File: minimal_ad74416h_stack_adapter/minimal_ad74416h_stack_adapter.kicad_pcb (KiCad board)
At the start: 2 copper layers, 5.1 x 5.1 mm, 0 parts

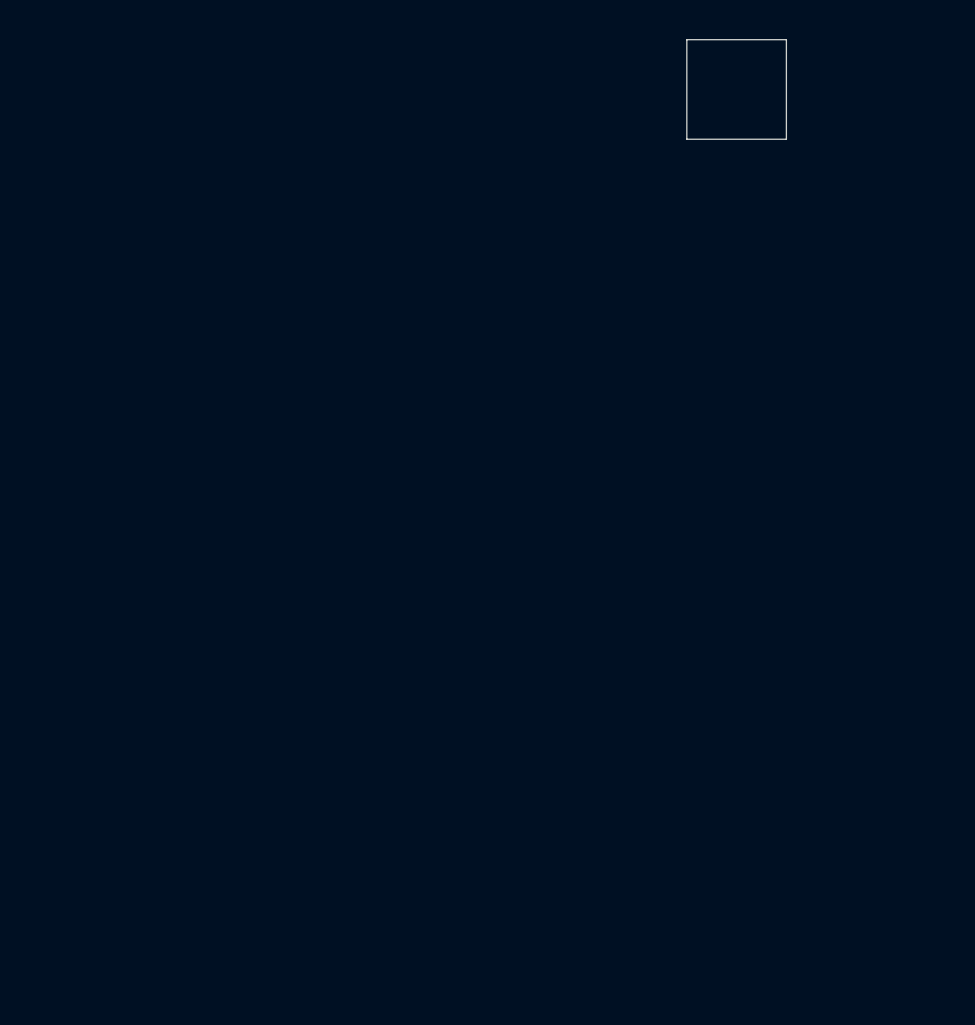
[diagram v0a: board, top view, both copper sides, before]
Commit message: backup
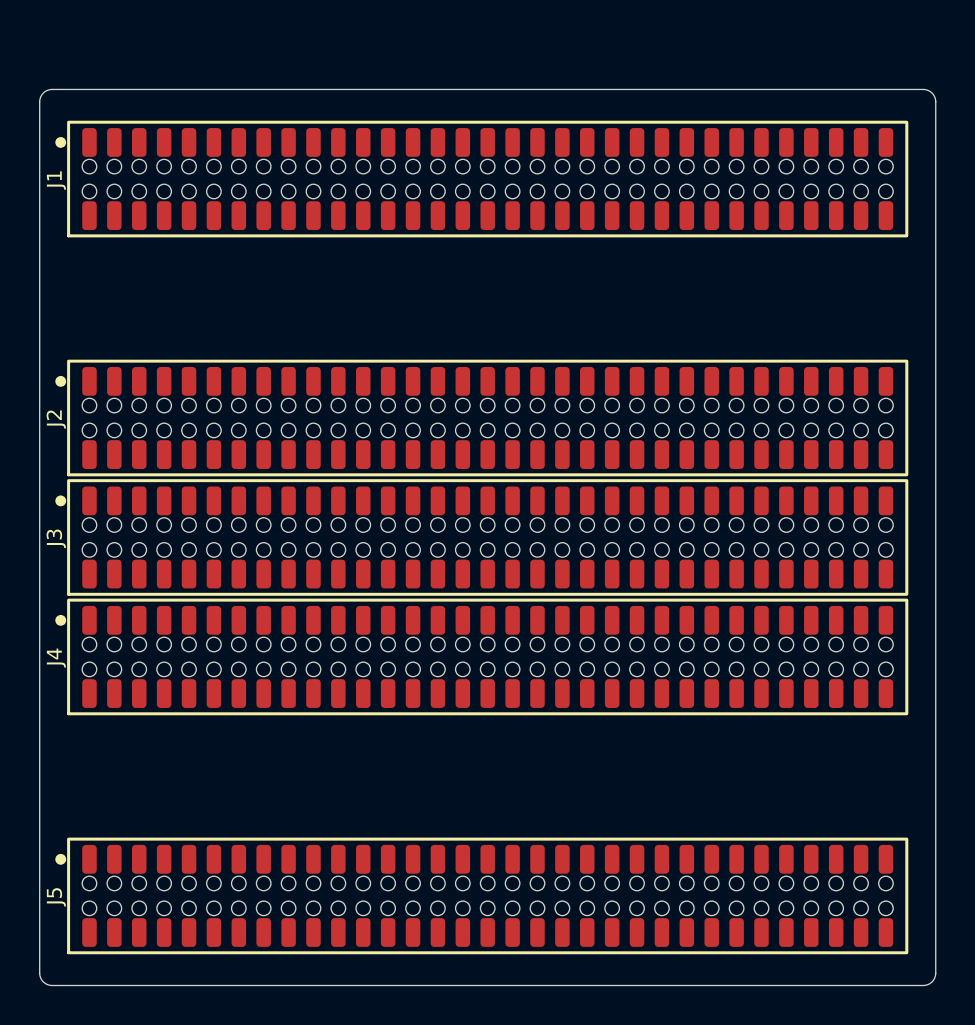
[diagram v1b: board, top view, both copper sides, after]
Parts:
- added J1: CLP-133-02-G-D-BE, connector_footprints:CLP-133-02-G-D-BE, F.Cu at (139.7, 106.2)
- added J2: CLP-133-02-G-D-BE, connector_footprints:CLP-133-02-G-D-BE, F.Cu at (139.7, 118.4)
- added J3: CLP-133-02-G-D-BE, connector_footprints:CLP-133-02-G-D-BE, F.Cu at (139.7, 124.5)
- added J4: CLP-133-02-G-D-BE, connector_footprints:CLP-133-02-G-D-BE, F.Cu at (139.7, 130.6)
- added J5: CLP-133-02-G-D-BE, connector_footprints:CLP-133-02-G-D-BE, F.Cu at (139.7, 142.7)
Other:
- board size 5.1 x 5.1 mm -> 45.7 x 45.7 mm
- copper layers 2 -> 4
